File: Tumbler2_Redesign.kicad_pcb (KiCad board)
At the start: 2 copper layers, 77 x 84 mm, 113 parts, among them J1 Conn_01x02, J2 Conn_01x05, J3 Conn_01x10, J4 Conn_01x10, J5 USB_C_Receptacle_USB2.0_16P, J6 USB_C_Receptacle_USB2.0_16P, J7 Conn_01x04, J8 Conn_01x06, J9 Conn_01x06, Q1 MMBT3904, Q3 MMBT3904, SW1 SW_Push, SW2 SW_Push, SW3 SW_Push, U1 CH340C, U11 TB6612FNG, U12 AMS1117-5.0, U2 LSM6DSV, U3 AP63203WU, U4 ESP32-S3-WROOM-1, U8 USBLC6-2SC6, U9 USBLC6-2SC6

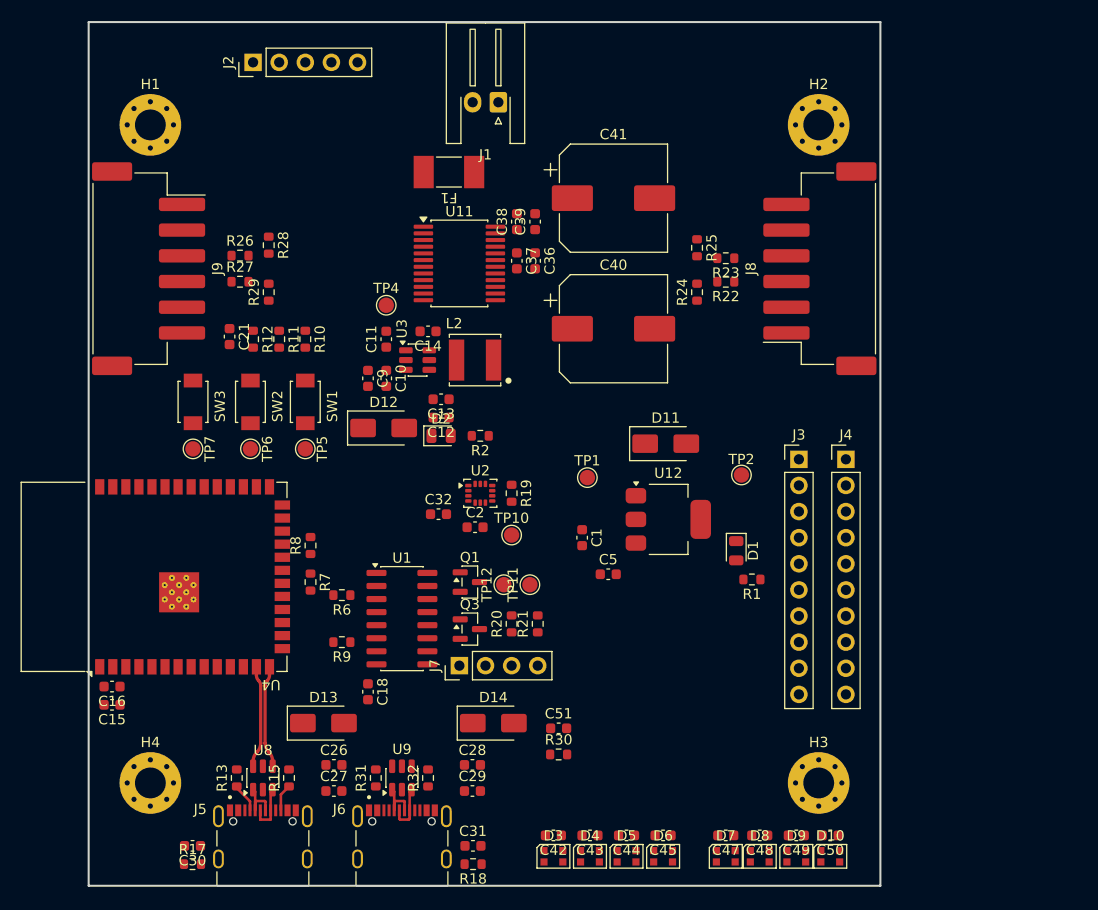
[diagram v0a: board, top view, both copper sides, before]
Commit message: Start conceptual layouting
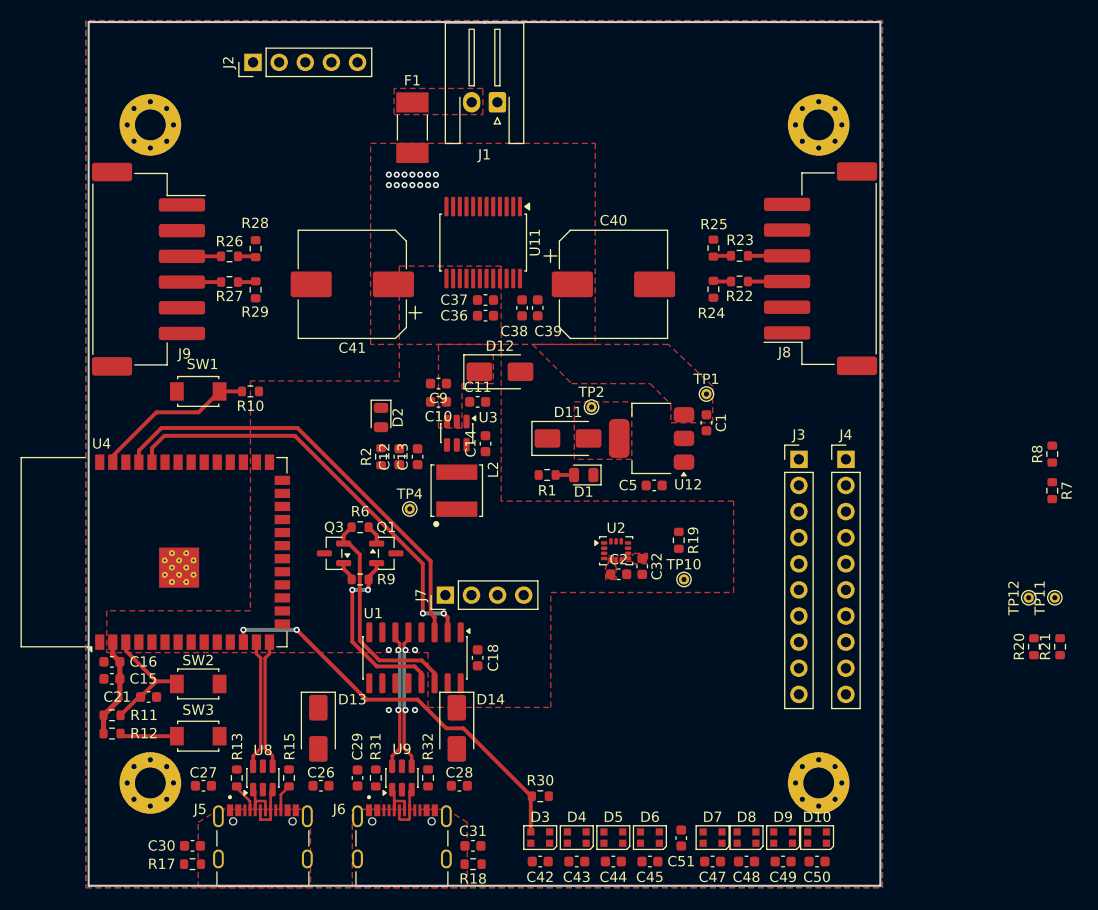
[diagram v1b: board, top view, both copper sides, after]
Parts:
- removed TP5, TP6, TP7: TestPoint, TestPoint:TestPoint_Pad_D1.5mm
- TP1, TP10, TP11, TP12, TP2, TP4: footprint TestPoint:TestPoint_Pad_D1.5mm -> TestPoint:TestPoint_THTPad_D1.0mm_Drill0.5mm
- moved R7 72.7 mm to (207.5, 106.9)
- moved R8 72.7 mm to (207.5, 103.4)
- moved TP11 51.1 mm to (207.8, 117.3)
- moved TP12 51.1 mm to (205.2, 117.3)
- moved R20 50.8 mm to (205.7, 122.1)
- moved R21 50.8 mm to (208.3, 122.1)
- moved R12 40.7 mm to (116.1, 130.6), turned to 0 degrees
- moved R11 40.0 mm to (116.1, 128.8), turned to 0 degrees
- moved C21 35.9 mm to (119.6, 127.0), turned to 0 degrees
- moved SW3 32.5 mm to (124.5, 130.8), turned to 180 degrees
- moved SW2 27.9 mm to (124.5, 125.7), turned to 180 degrees
- moved C41 26.7 mm to (139.4, 86.9), turned to 180 degrees
- moved R1 22.4 mm to (158.4, 105.4), turned to 0 degrees
- moved C32 20.5 mm to (167.6, 114.3), turned to -90 degrees
- moved TP4 19.9 mm to (145.0, 108.7)
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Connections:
- net /Peripherals/M1_M renamed /Peripherals/M1_N
- net /Peripherals/M2_M renamed /Peripherals/M2_N
- U4 pad 12: /MCU/IO8 -> /MCU/RGB
- U4 pad 23: /MCU/RGB -> /MCU/IO8
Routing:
- net /MCU/TXD: track 0.00 -> 42.9 mm
- net /MCU/RXD: track 0.00 -> 42.2 mm, vias 0 -> 2
- net /MCU/RGB: track 0.00 -> 39.4 mm, vias 0 -> 2
- net /MCU/RTS: track 0.00 -> 21.9 mm
- net /MCU/DTR: track 0.00 -> 18.5 mm, vias 0 -> 2
- net /MCU/BTN: track 0.00 -> 15.8 mm
- net /MCU/DP_2: track 0.00 -> 13.7 mm, vias 0 -> 2
- net /MCU/DN_2: track 0.00 -> 13.7 mm, vias 0 -> 2
- net /MCU/ENABLE: track 0.00 -> 12.0 mm
- net 3.3V: track 0.00 -> 9.83 mm
- net /MCU/GPIO0: track 0.00 -> 5.59 mm
- net Net-(J8-Pin_4): track 0.00 -> 3.81 mm
- net Net-(J8-Pin_3): track 0.00 -> 3.81 mm
- net Net-(J9-Pin_4): track 0.00 -> 3.80 mm
- net Net-(J9-Pin_3): track 0.00 -> 3.80 mm
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- added copper zone on F.Cu, net 3.3V
- added copper zone on B.Cu, net GND
- added copper zone on F.Cu, net GND
- added copper zone on F.Cu, net Net-(D11-A)
- added copper zone on F.Cu, net Net-(J1-Pin_2)
- added copper zone on F.Cu, net Net-(J5-SHIELD)
- added copper zone on F.Cu, net Net-(J6-SHIELD)
- added copper zone on F.Cu, net VBAT
